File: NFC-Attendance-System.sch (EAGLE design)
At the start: 14 parts, among them J1 NFC_HDR, J2 DAC_HDR, J3 LCD_HDR, Q1 8550, SW1 PROG, SW2 RST, U1 ESP-WROOM-32

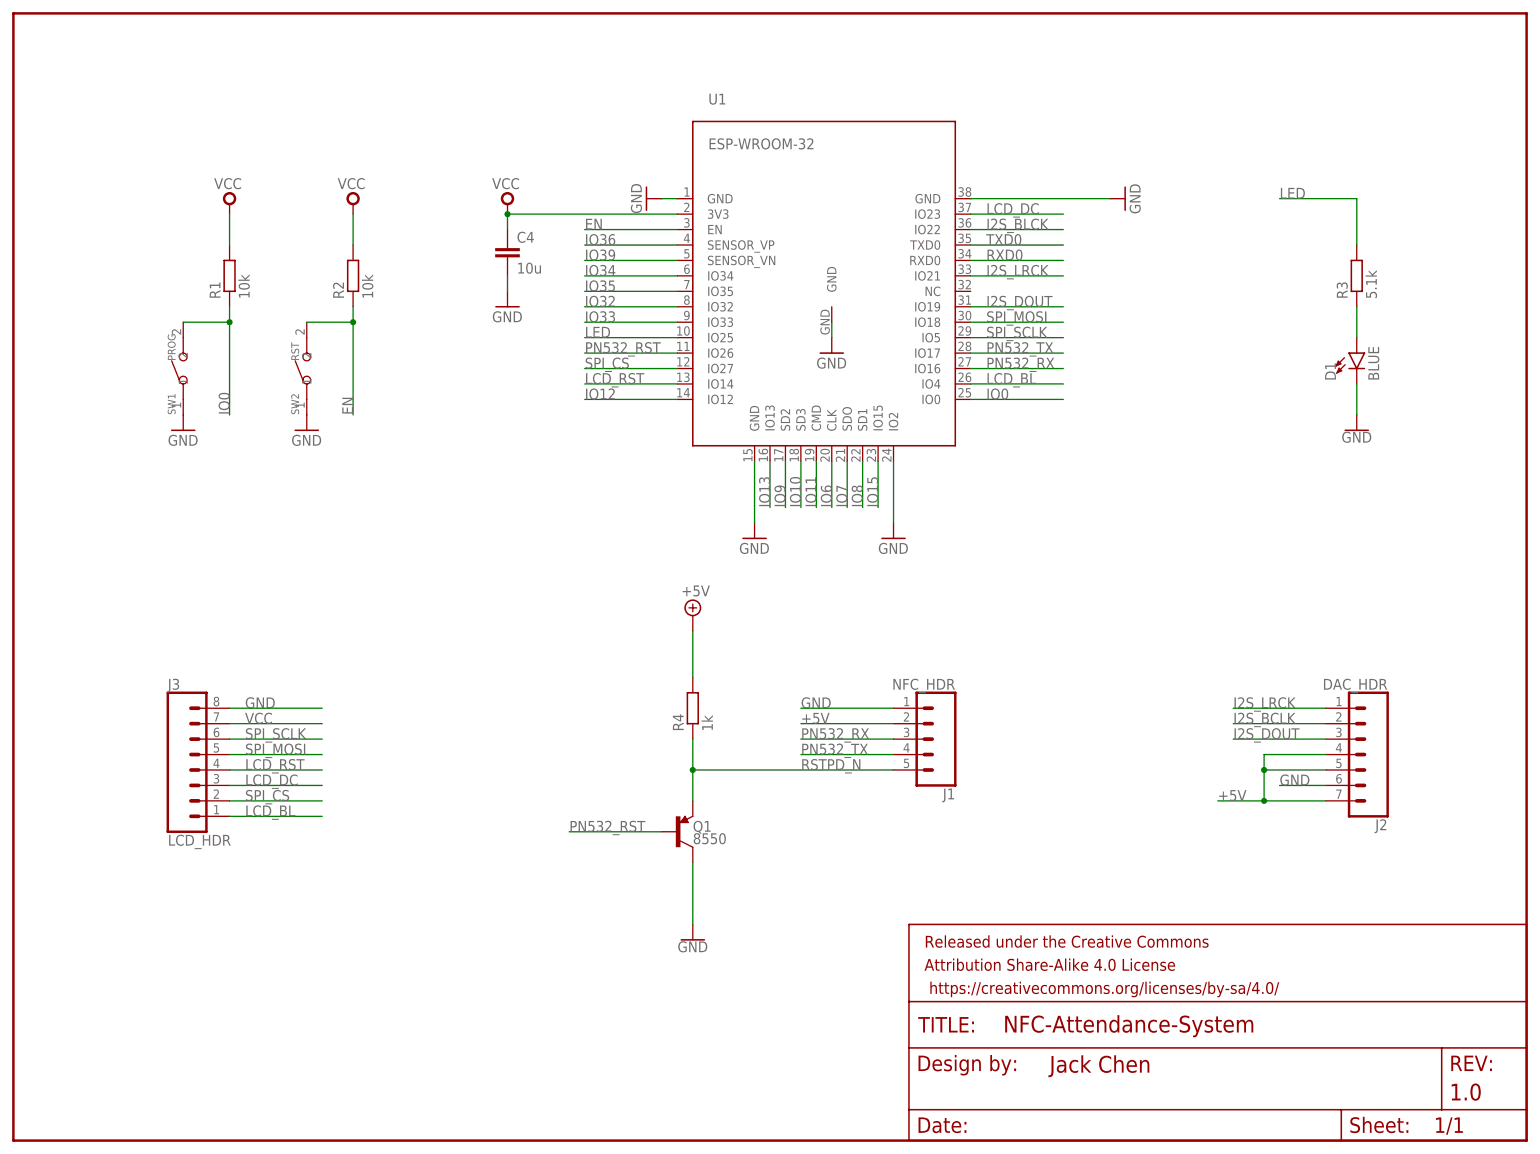
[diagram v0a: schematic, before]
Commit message: minor fixes
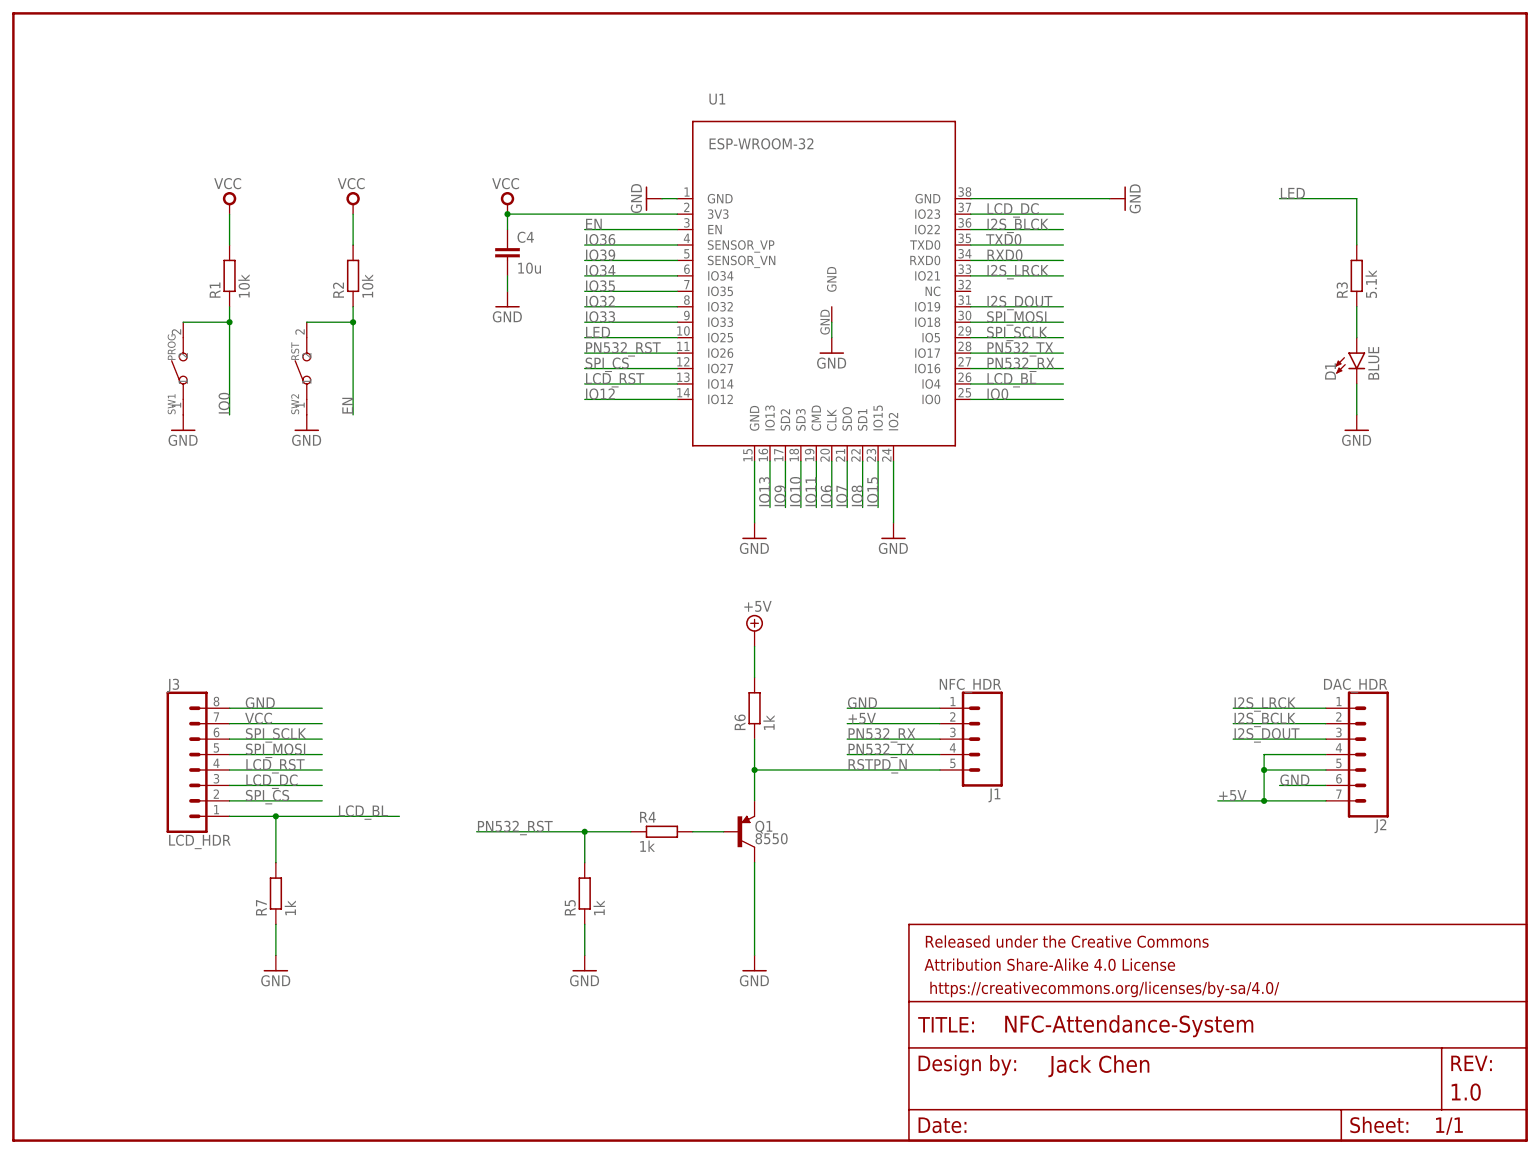
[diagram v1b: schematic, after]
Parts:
- added R5, R6, R7: 1k, rcl:R-EU_R0603
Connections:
- new net N$2: Q1.B, R4.2
- net +5V: now also R6.2; no longer R4.2
- net GND: now also R5.1, R7.1
- net LCD_BL: now also R7.2
- net PN532_RST: now also R4.1, R5.2; no longer Q1.B
- net RSTPD_N: now also R6.1; no longer R4.1
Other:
- moved on the sheet: J1, Q1, R4
